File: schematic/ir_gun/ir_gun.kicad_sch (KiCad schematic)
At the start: 8 parts, among them Q1 2SC1815, SW1 Attack, SW2 Reload

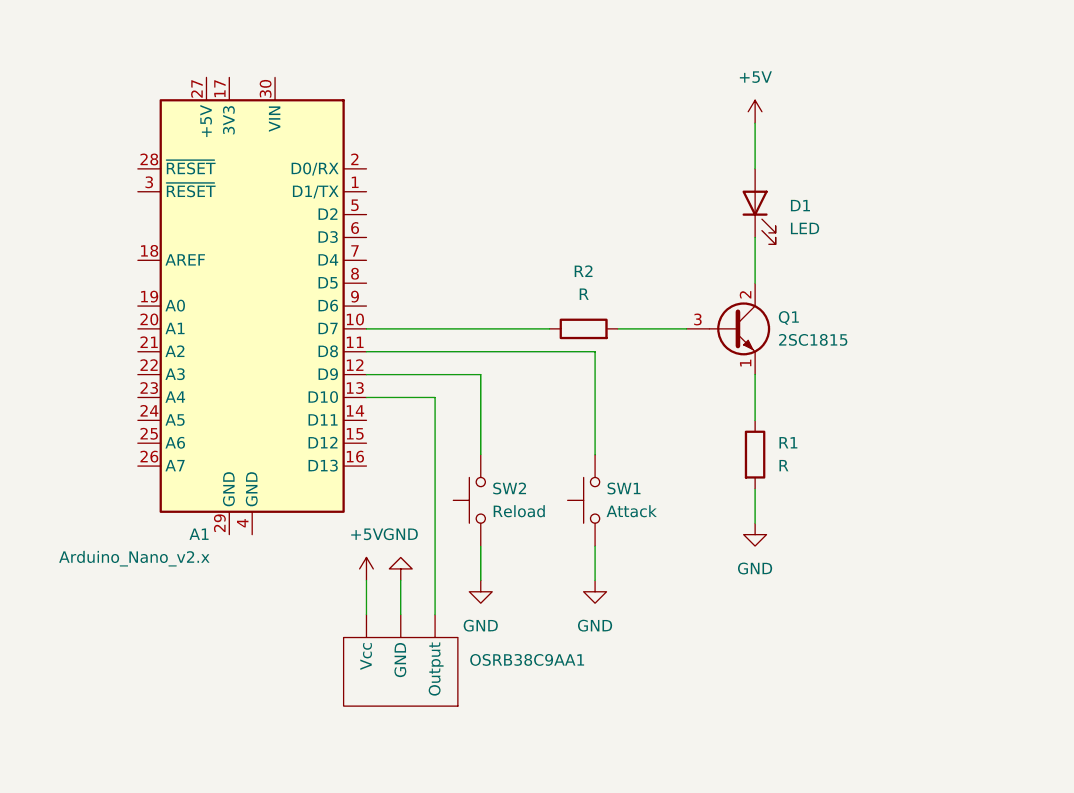
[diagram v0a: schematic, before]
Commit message: ✨ 回路図を追加
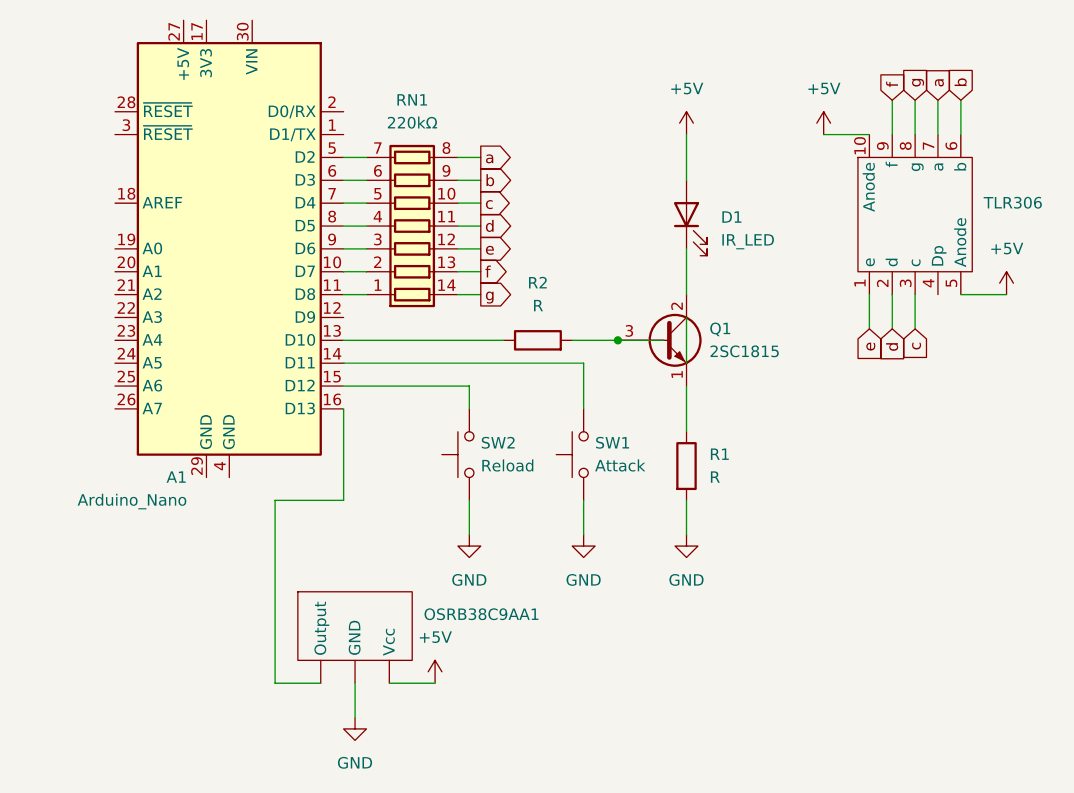
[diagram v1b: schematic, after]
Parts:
- added RN1: 220kΩ, symbol Device:R_Pack07
- added TLR306: ~, symbol tlr306:tlr306
- A1: value Arduino_Nano_v2.x -> Arduino_Nano
- D1: value LED -> IR_LED
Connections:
- net +5V: now also TLR306.10 (Anode), TLR306.5 (Anode)
- net at A1.13 (D10): now also R2.1; no longer OSRB38C9AA1. (Vcc)
- net at A1.10 (D7): now also RN1.2 (R2.1); no longer R2.1
- net at A1.11 (D8): now also RN1.1 (R1.1); no longer SW1.2
- net at A1.12 (D9): no longer SW2.2
- net at A1.14 (D11): now also SW1.2
- net at A1.15 (D12): now also SW2.2
- net at A1.16 (D13): now also OSRB38C9AA1. (Vcc)
- net at A1.5 (D2): now also RN1.7 (R7.1)
- net at A1.6 (D3): now also RN1.6 (R6.1)
- net at A1.7 (D4): now also RN1.5 (R5.1)
- net at A1.8 (D5): now also RN1.4 (R4.1)
- net at A1.9 (D6): now also RN1.3 (R3.1)
- new net a: RN1.8 (R7.2), TLR306.7 (a)
- new net b: RN1.9 (R6.2), TLR306.6 (b)
- new net c: RN1.10 (R5.2), TLR306.3 (c)
- new net d: RN1.11 (R4.2), TLR306.2 (d)
- new net e: RN1.12 (R3.2), TLR306.1 (e)
- new net f: RN1.13 (R2.2), TLR306.9 (f)
- new net g: RN1.14 (R1.2), TLR306.8 (g)
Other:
- moved on the sheet: A1, D1, OSRB38C9AA1, Q1, R1, R2, SW1, SW2
